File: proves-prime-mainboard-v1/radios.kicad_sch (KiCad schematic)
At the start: 12 parts, among them J10 Conn_Coaxial, J9 Conn_Coaxial, U10 RFM9xBreakout, U7 RFM98PW, U8 RFM9xBreakout, U9 RFM98PW

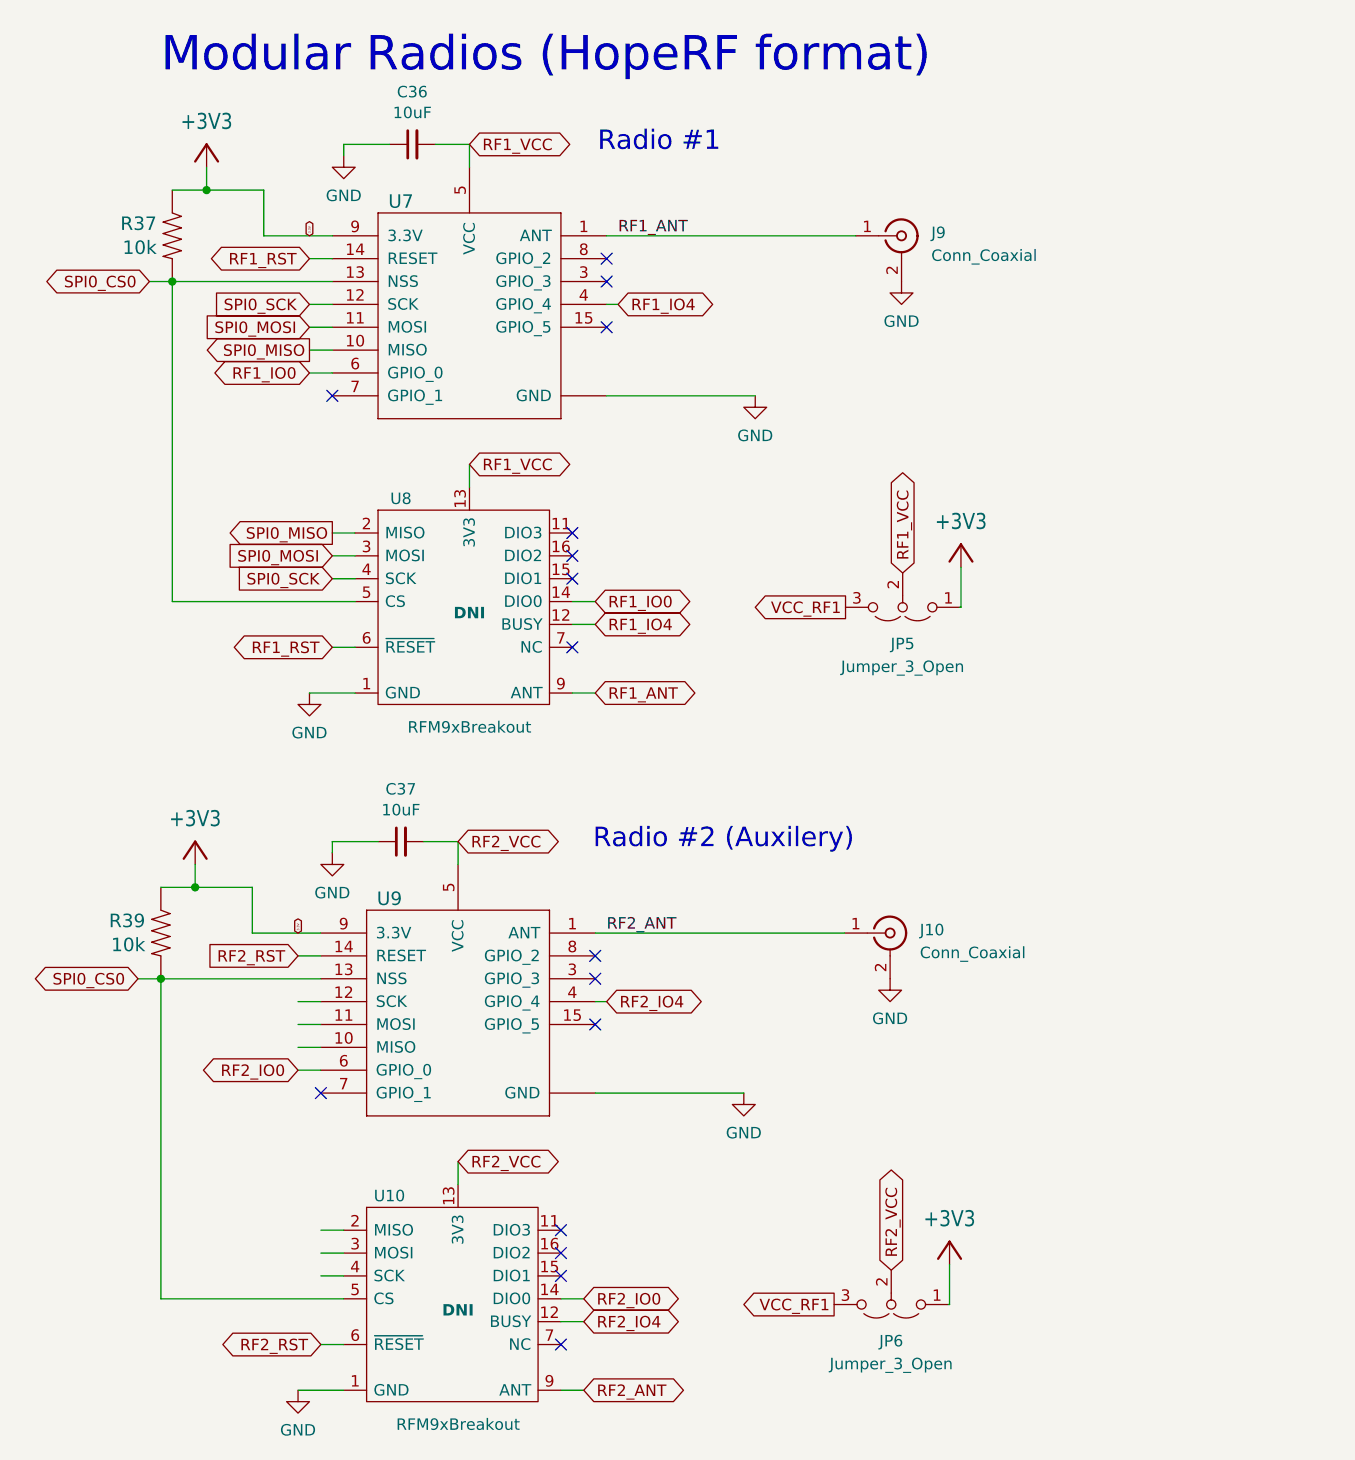
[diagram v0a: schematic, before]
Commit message: Removed Unneeded Stuff
- Took away small RFM footprint from Radio 1
- Removed the cursed CAN bus
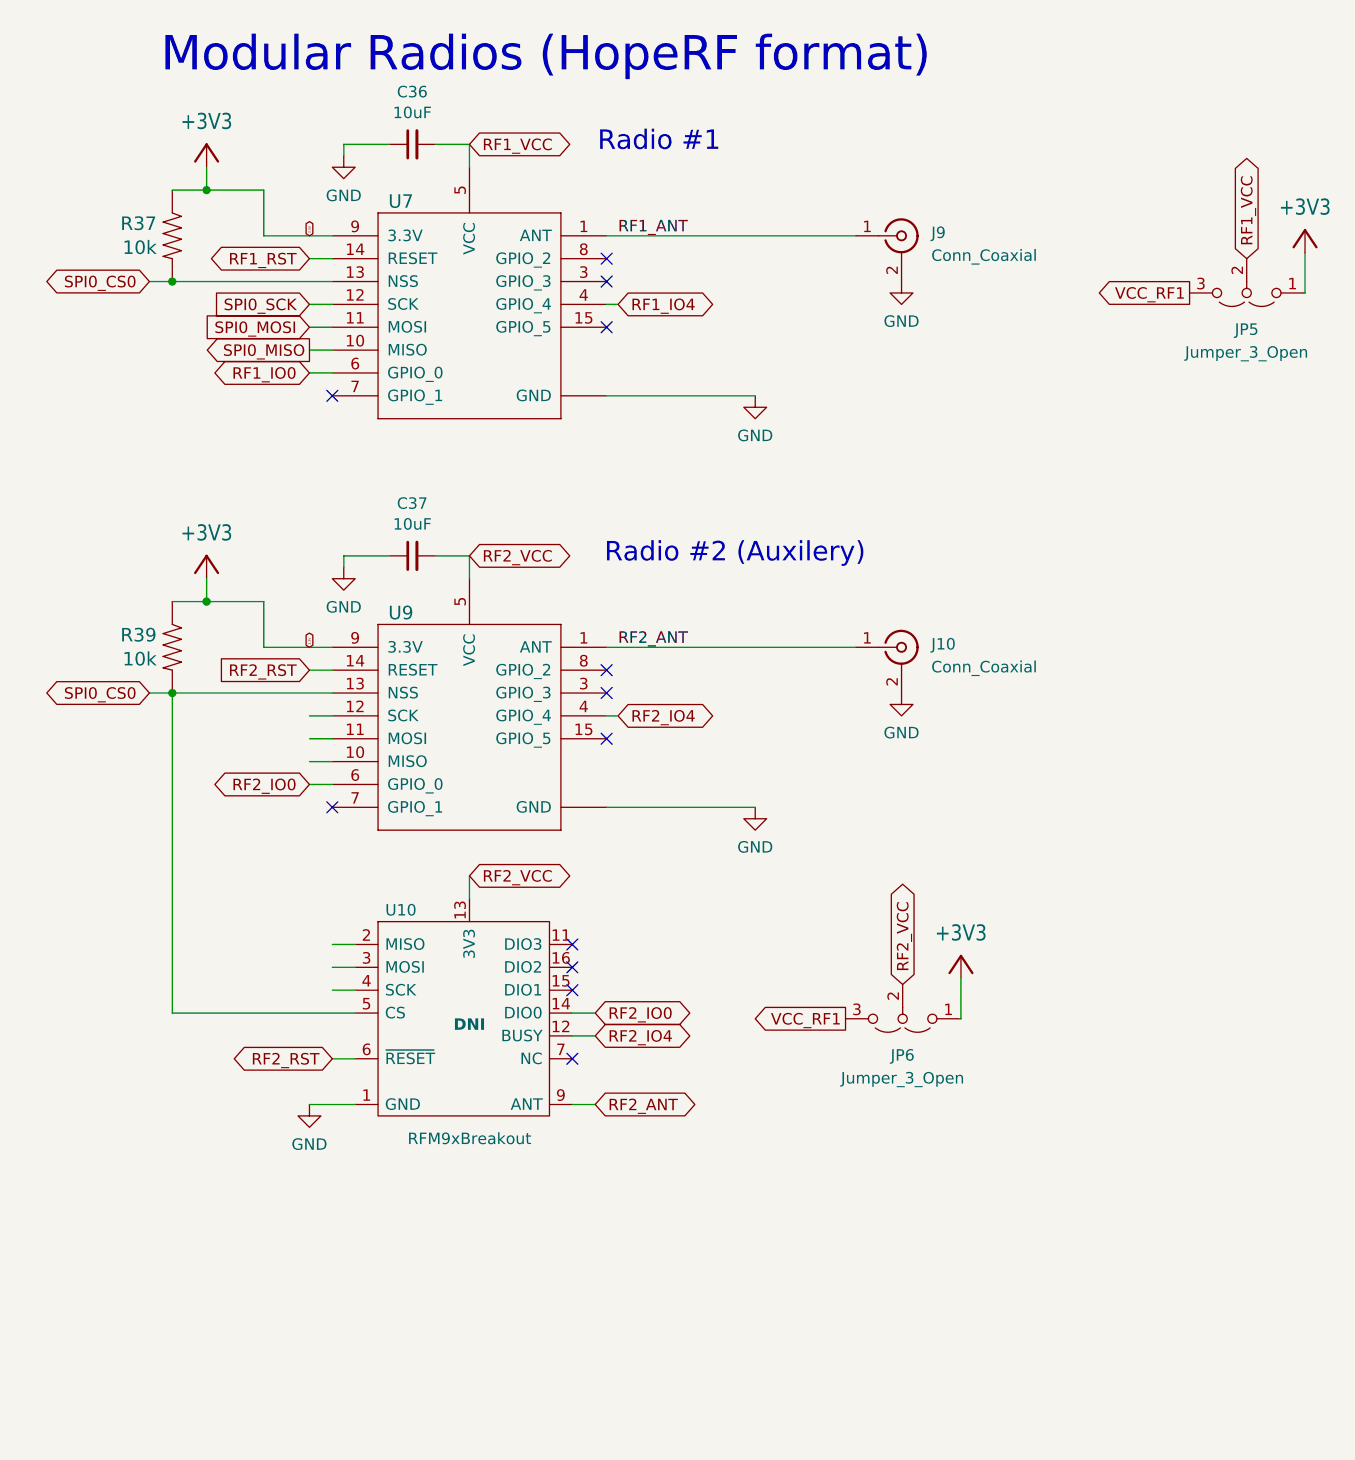
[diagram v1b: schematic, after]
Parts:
- removed U8: RFM9xBreakout, RF_Module:HOPERF_RFM9XW_SMD, symbol mainboard:RFM9xBreakout
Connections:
- no-connect marks 16 -> 12
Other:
- moved on the sheet: C37, J10, JP5, JP6, R39, U10, U9
